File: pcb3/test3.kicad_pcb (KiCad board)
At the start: 2 copper layers, 52 parts, among them CON1 BARREL_JACK, CON2 BARREL_JACK, IC1 ATMEGA8A-A, P1 USB_A, SW1 SW_PUSH

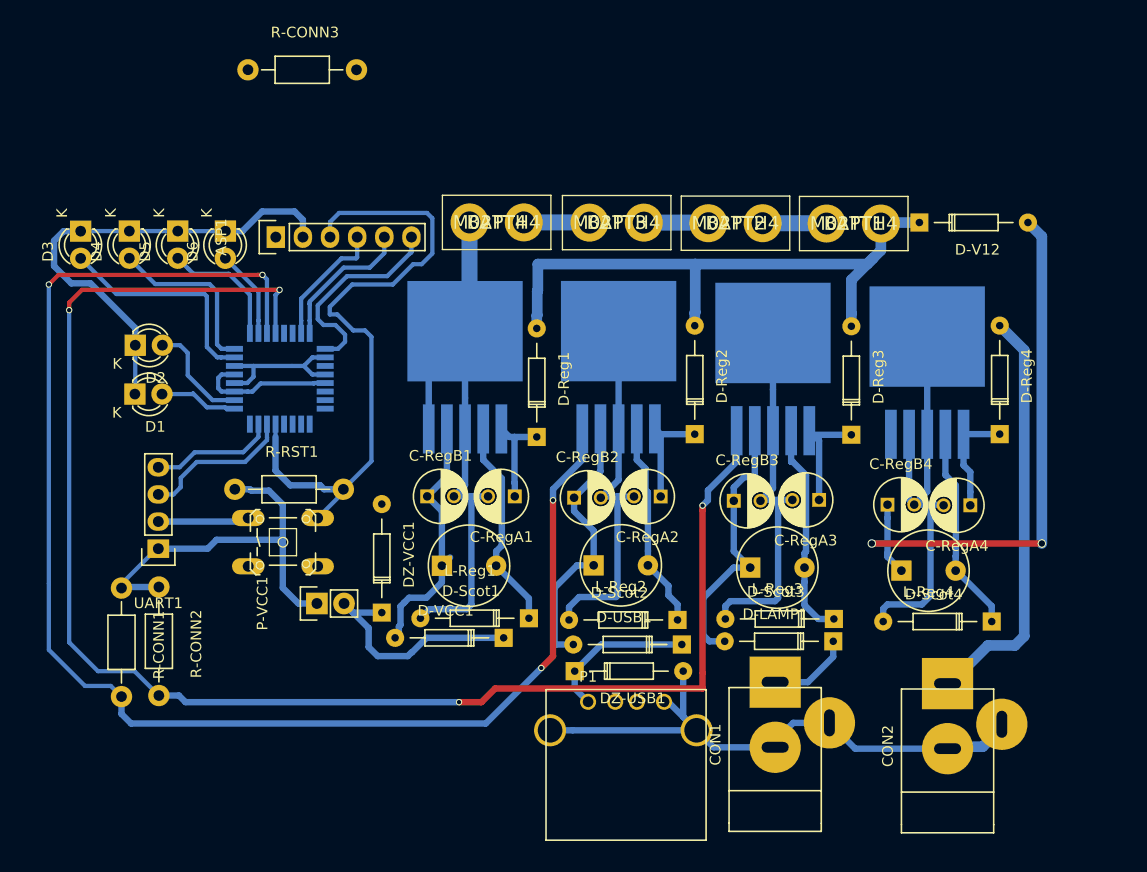
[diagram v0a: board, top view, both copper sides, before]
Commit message: belum apply revisi
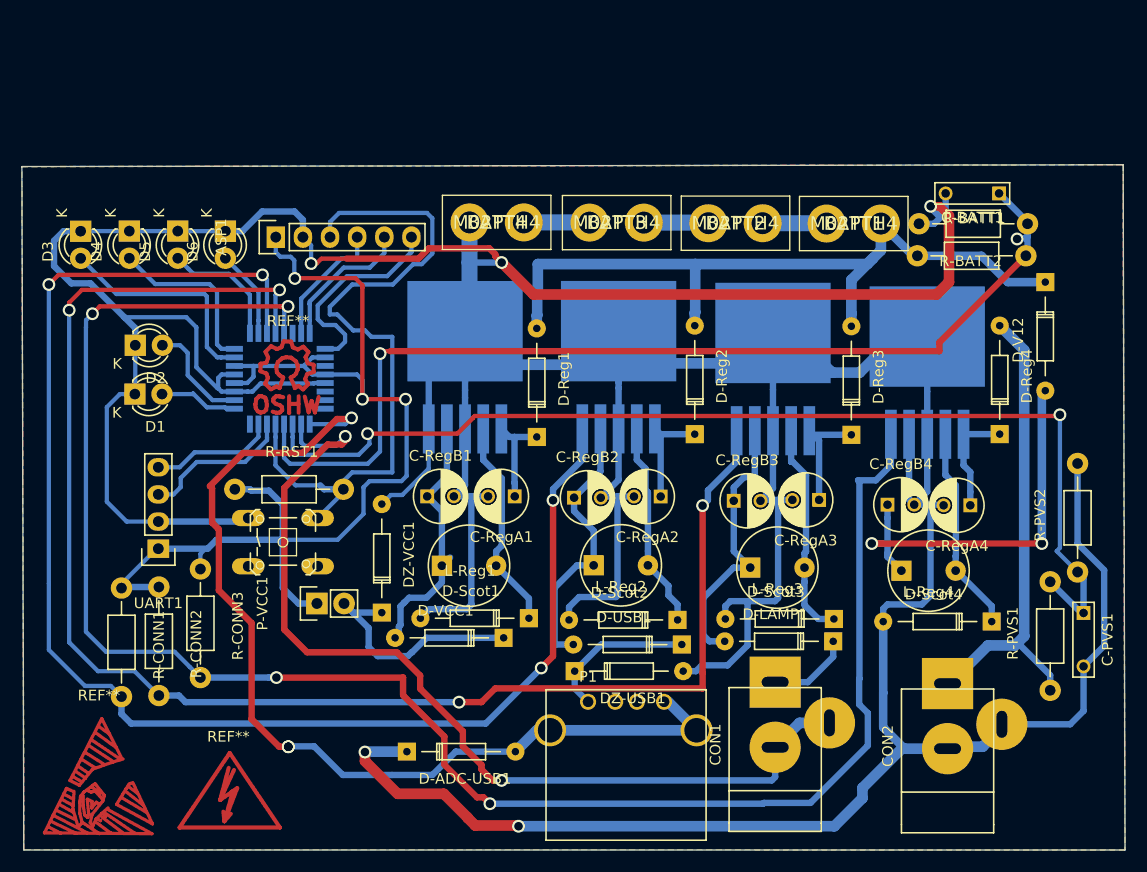
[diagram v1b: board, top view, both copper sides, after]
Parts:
- added C-BATT1: C, Capacitors_ThroughHole:C_Rect_L7_W2_P5, F.Cu at (193.2, 68.8)
- added C-PVS1: C, Capacitors_ThroughHole:C_Rect_L7_W2_P5, F.Cu at (201.1, 108.1)
- added D-ADC-USB1: D, Diodes_ThroughHole:Diode_DO-35_SOD27_Horizontal_RM10, F.Cu at (137.7, 121.0)
- added R-BATT1: R, Resistors_ThroughHole:Resistor_Horizontal_RM10mm, F.Cu at (190.6, 74.6)
- added R-BATT2: R, Resistors_ThroughHole:Resistor_Horizontal_RM10mm, F.Cu at (190.7, 71.6)
- added R-PVS1: R, Resistors_ThroughHole:Resistor_Horizontal_RM10mm, F.Cu at (197.9, 110.2)
- added R-PVS2: R, Resistors_ThroughHole:Resistor_Horizontal_RM10mm, F.Cu at (200.5, 99.1)
- added REF**: Symbol_ESD-Logo_CopperTop, Symbols:Symbol_ESD-Logo_CopperTop, F.Cu at (108.9, 125.3)
- added REF**: Symbol_HighVoltage_Type2_CopperTop_VerySmall, Symbols:Symbol_HighVoltage_Type2_CopperTop_VerySmall, F.Cu at (121.1, 125.3)
- added REF**: Symbol_OSHW-Logo_CopperTop, Symbols:Symbol_OSHW-Logo_CopperTop, F.Cu at (126.5, 85.1)
- moved R-CONN3 52.7 mm to (118.4, 109.0), turned to 270 degrees
- moved D-V12 13.0 mm to (197.5, 77.1), turned to 270 degrees
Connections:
- net Net-(CON2-Pad1) renamed /PV-IN
- CON1 pad 2: GND -> /ADC-LAMP
- CON1 pad 3: GND -> /ADC-LAMP
- IC-Reg4 pad 5: Net-(IC-Reg4-Pad5) -> /CONN-PV
- IC1 pad 25: Net-(IC1-Pad25) -> /ADC-USB
- IC1 pad 26: Net-(IC1-Pad26) -> /ADC-LAMP
- IC1 pad 27: Net-(IC1-Pad27) -> /ADC-PV
- IC1 pad 28: Net-(IC1-Pad28) -> /ADC-BATT
- P1 pad 4: GND -> /ADC-USB
- P1 pad 5: GND -> /ADC-USB
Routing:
- net GND: track 288.9 -> 536.8 mm, vias 0 -> 5
- net /CONN-PV: track 0.00 -> 167.7 mm, vias 0 -> 4
- net /ADC-PV: track 0.00 -> 101.1 mm, vias 0 -> 2
- net /ADC-BATT: track 0.00 -> 94.8 mm, vias 0 -> 2
- net /ADC-USB: track 0.00 -> 93.2 mm, vias 0 -> 3
- net /ADC-LAMP: track 0.00 -> 90.9 mm, vias 0 -> 2
- net VCC: track 51.7 -> 108.8 mm, vias 0 -> 3
- net Net-(C-RegB4-Pad1): track 55.0 -> 38.9 mm
- net +12V: track 57.9 -> 74.0 mm
- net /PV-IN: track 39.0 -> 44.9 mm
- net /NRST: track 63.2 -> 67.9 mm
- added copper zone on B.Cu, net (none)
- added copper zone on F.Cu, net (none)
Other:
- board outline added: 103.3 x 64.1 mm
- net class Default: via_dia 0.6 -> 1.2; via_drill 0.4 -> 0.8
